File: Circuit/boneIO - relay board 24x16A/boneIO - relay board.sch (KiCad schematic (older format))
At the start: 67 parts, among them J1 Screw_Terminal_01x04, J10 Screw_Terminal_01x04, J11 Screw_Terminal_01x04, J12 Screw_Terminal_01x04, J13 Screw_Terminal_01x04, J2 Screw_Terminal_01x04, J3 Conn_02x04_Odd_Even, J4 Screw_Terminal_01x04, J5 Screw_Terminal_01x04, J6 Screw_Terminal_01x04, J7 Screw_Terminal_01x04, J8 Screw_Terminal_01x04, J9 Screw_Terminal_01x04, K1 RM85-2011-35-1024, K10 RM85-2011-35-1024, K11 RM85-2011-35-1024, K12 RM85-2011-35-1024, K13 RM85-2011-35-1024, K14 RM85-2011-35-1024, K15 RM85-2011-35-1024, K16 RM85-2011-35-1024, K17 RM85-2011-35-1024, K18 RM85-2011-35-1024, K19 RM85-2011-35-1024, K2 RM85-2011-35-1024, K20 RM85-2011-35-1024, K21 RM85-2011-35-1024, K22 RM85-2011-35-1024, K23 RM85-2011-35-1024, K24 RM85-2011-35-1024, K3 RM85-2011-35-1024, K4 RM85-2011-35-1024, K5 RM85-2011-35-1024, K6 RM85-2011-35-1024, K7 RM85-2011-35-1024, K8 RM85-2011-35-1024, K9 RM85-2011-35-1024, SW1 SW_DIP_x03, SW2 SW_DIP_x03, SW3 SW_DIP_x03, U1 MCP9808_MSOP, U2 MCP23017_SS, U3 MCP23017_SS, U4 ULN2803A, U5 ULN2803A, U6 ULN2803A

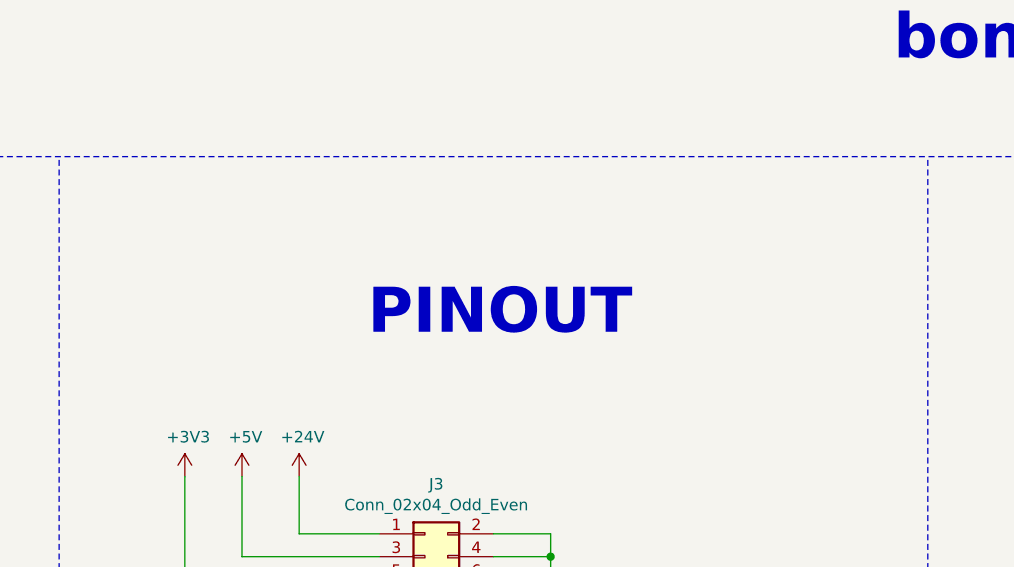
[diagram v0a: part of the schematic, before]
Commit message: correcting the scheme
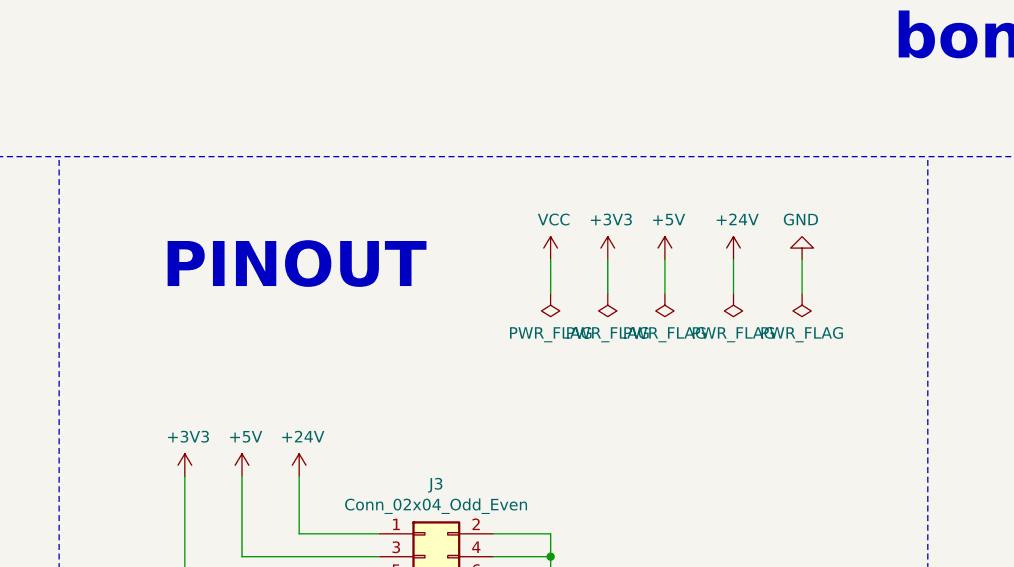
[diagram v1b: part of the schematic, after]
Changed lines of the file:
@@
 Wire Wire Line
 	18050 13550 18250 13550
-Text Notes 6100 2400 0    197  ~ 39
+Text Notes 5200 2200 0    197  ~ 39
 PINOUT
 Text Notes 11500 2350 0    197  ~ 39
@@
 	21700 2250 21700 2500
 Connection ~ 21700 2500
+$Comp
+L power:PWR_FLAG #FLG0101
+U 1 1 619EE2AC
+P 7150 2200
+F 0 "#FLG0101" H 7150 2275 50  0001 C CNN
+F 1 "PWR_FLAG" H 7150 2373 50  0000 C CNN
+F 2 "" H 7150 2200 50  0001 C CNN
+F 3 "~" H 7150 2200 50  0001 C CNN
+	1    7150 2200
+	-1   0    0    1
+$EndComp
+$Comp
+L power:+3V3 #PWR0133
+U 1 1 619EE9F3
+P 7150 2050
+F 0 "#PWR0133" H 7150 1900 50  0001 C CNN
+F 1 "+3V3" H 7165 2223 50  0000 C CNN
+F 2 "" H 7150 2050 50  0001 C CNN
+F 3 "" H 7150 2050 50  0001 C CNN
+	1    7150 2050
+	1    0    0    -1
+$EndComp
+Wire Wire Line
+	7150 2200 7150 2050
+$Comp
+L power:+5V #PWR0134
+U 1 1 61AA15B4
+P 7400 2050
+F 0 "#PWR0134" H 7400 1900 50  0001 C CNN
+F 1 "+5V" H 7415 2223 50  0000 C CNN
+F 2 "" H 7400 2050 50  0001 C CNN
+F 3 "" H 7400 2050 50  0001 C CNN
+	1    7400 2050
+	1    0    0    -1
+$EndComp
+$Comp
+L power:PWR_FLAG #FLG0102
+U 1 1 61ADCEBD
+P 7400 2200
+F 0 "#FLG0102" H 7400 2275 50  0001 C CNN
+F 1 "PWR_FLAG" H 7400 2373 50  0000 C CNN
+F 2 "" H 7400 2200 50  0001 C CNN
+F 3 "~" H 7400 2200 50  0001 C CNN
+	1    7400 2200
+	-1   0    0    1
+$EndComp
+Wire Wire Line
+	7400 2200 7400 2050
+$Comp
+L power:+24V #PWR0135
+U 1 1 61B18DCF
+P 7700 2050
+F 0 "#PWR0135" H 7700 1900 50  0001 C CNN
+F 1 "+24V" H 7715 2223 50  0000 C CNN
+F 2 "" H 7700 2050 50  0001 C CNN
+F 3 "" H 7700 2050 50  0001 C CNN
+	1    7700 2050
+	1    0    0    -1
+$EndComp
+$Comp
+L power:PWR_FLAG #FLG0103
+U 1 1 61B54C9F
+P 7700 2200
+F 0 "#FLG0103" H 7700 2275 50  0001 C CNN
+F 1 "PWR_FLAG" H 7700 2373 50  0000 C CNN
+F 2 "" H 7700 2200 50  0001 C CNN
+F 3 "~" H 7700 2200 50  0001 C CNN
+	1    7700 2200
+	-1   0    0    1
+$EndComp
+Wire Wire Line
+	7700 2200 7700 2050
+$Comp
+L power:GND #PWR0136
+U 1 1 61BCD558
+P 8000 2050
+F 0 "#PWR0136" H 8000 1800 50  0001 C CNN
+F 1 "GND" H 8005 1877 50  0000 C CNN
+F 2 "" H 8000 2050 50  0001 C CNN
+F 3 "" H 8000 2050 50  0001 C CNN
+	1    8000 2050
+	-1   0    0    1
+$EndComp
+Wire Wire Line
+	8000 2200 8000 2050
+$Comp
+L power:VCC #PWR0137
+U 1 1 61CFBC73
+P 6900 2050
+F 0 "#PWR0137" H 6900 1900 50  0001 C CNN
+F 1 "VCC" H 6915 2223 50  0000 C CNN
+F 2 "" H 6900 2050 50  0001 C CNN
+F 3 "" H 6900 2050 50  0001 C CNN
+	1    6900 2050
+	1    0    0    -1
+$EndComp
+$Comp
+L power:PWR_FLAG #FLG0104
+U 1 1 61D38686
+P 6900 2200
+F 0 "#FLG0104" H 6900 2275 50  0001 C CNN
+F 1 "PWR_FLAG" H 6900 2373 50  0000 C CNN
+F 2 "" H 6900 2200 50  0001 C CNN
+F 3 "~" H 6900 2200 50  0001 C CNN
+	1    6900 2200
+	-1   0    0    1
+$EndComp
+Wire Wire Line
+	6900 2200 6900 2050
+$Comp
+L power:PWR_FLAG #FLG0105
+U 1 1 61DB26DF
+P 8000 2200
+F 0 "#FLG0105" H 8000 2275 50  0001 C CNN
+F 1 "PWR_FLAG" H 8000 2373 50  0000 C CNN
+F 2 "" H 8000 2200 50  0001 C CNN
+F 3 "~" H 8000 2200 50  0001 C CNN
+	1    8000 2200
+	-1   0    0    1
+$EndComp
 $EndSCHEMATC
